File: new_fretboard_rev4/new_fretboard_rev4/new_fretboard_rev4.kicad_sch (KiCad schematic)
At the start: 48 parts, among them J1 Conn_01x06, J2 Conn_01x06, U1 LX3302AQPW_TSSOP-14, U2 LX3302AQPW_TSSOP-14

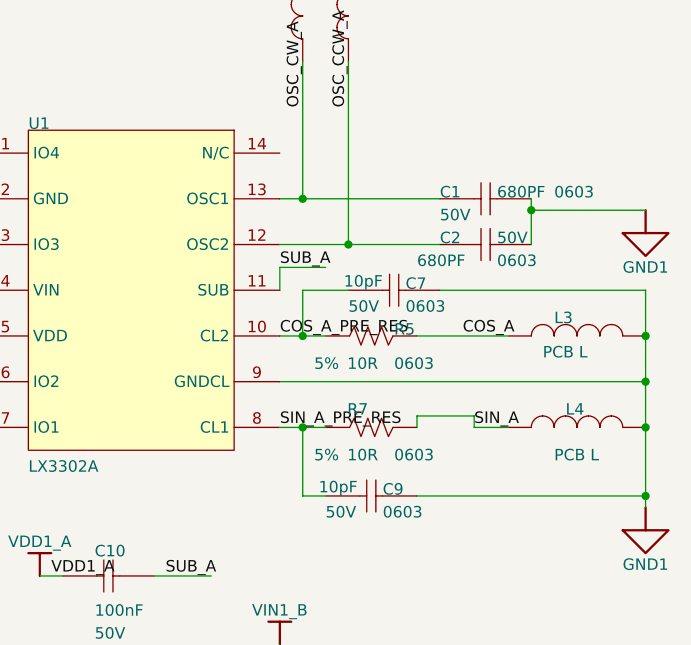
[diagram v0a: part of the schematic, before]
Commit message: partway through routing top
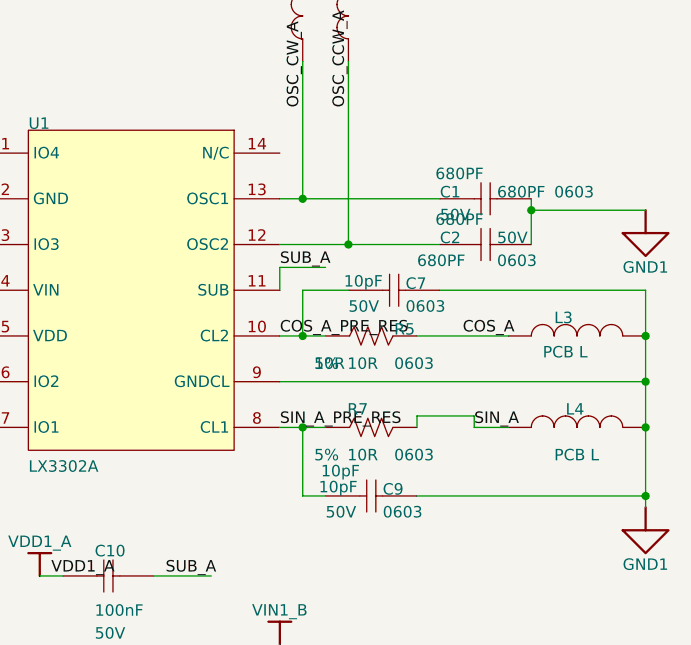
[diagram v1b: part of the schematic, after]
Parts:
- C1, C2, C21, C22: value Capacitor NP -> 680PF
- C10, C14, C18, C8: value Capacitor NP -> 100nF
- C11, C12, C13, C6: value Capacitor NP -> 6.8nF
- C15, C3: value Capacitor NP -> 1000pF
- C16, C4: value Capacitor NP -> 470nF
- C17, C5: value Capacitor NP -> 1uF
- C19, C20, C7, C9: value Capacitor NP -> 10pF
- R1, R8: value Resistor -> 221R
- R10, R2, R4, R9: value Resistor -> 10k
- R11, R6: value Resistor -> 4.7R
- R12, R13, R14, R3, R5, R7: value Resistor -> 10R
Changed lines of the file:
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@@
 			)
 		)
-		(property "Value" "Capacitor NP"
+		(property "Value" "680PF"
 			(at 200.152 76.708 0)
 			(effects
@@
 				)
 				(justify left bottom)
-				(hide yes)
 			)
 		)
@@
 			)
 		)
-		(property "Value" "Capacitor NP"
+		(property "Value" "6.8nF"
 			(at 53.848 184.912 0)
 			(effects
@@
 			)
 		)
-		(property "Value" "Capacitor NP"
+		(property "Value" "470nF"
 			(at 124.968 102.108 0)
 			(effects
@@
 			)
 		)
-		(property "Value" "Resistor"
+		(property "Value" "10R"
 			(at 184.15 203.2 0)
 			(effects
@@
 			)
 		)
-		(property "Value" "Capacitor NP"
+		(property "Value" "1uF"
 			(at 140.208 102.362 0)
 			(effects
@@
 			)
 		)
-		(property "Value" "Resistor"
+		(property "Value" "10k"
 			(at 96.52 75.692 0)
 			(effects
@@
 			)
 		)
-		(property "Value" "Capacitor NP"
+		(property "Value" "100nF"
 			(at 155.702 213.868 0)
 			(effects
@@
 			)
 		)
-		(property "Value" "Capacitor NP"
+		(property "Value" "6.8nF"
 			(at 76.708 184.912 0)
 			(effects
@@
 			)
 		)
-		(property "Value" "Capacitor NP"
+		(property "Value" "100nF"
 			(at 89.408 102.362 0)
 			(effects
@@
 			)
 		)
-		(property "Value" "Capacitor NP"
+		(property "Value" "6.8nF"
 			(at 56.388 89.662 0)
 			(effects
@@
 			)
 		)
-		(property "Value" "Capacitor NP"
+		(property "Value" "680PF"
 			(at 197.612 177.038 0)
 			(effects
@@
 			)
 		)
-		(property "Value" "Capacitor NP"
+		(property "Value" "6.8nF"
 			(at 79.248 89.662 0)
 			(effects
@@
 			)
 		)
-		(property "Value" "Resistor"
+		(property "Value" "4.7R"
 			(at 96.52 201.93 0)
 			(effects
@@
 			)
 		)
-		(property "Value" "Capacitor NP"
+		(property "Value" "10pF"
 			(at 189.992 86.868 0)
 			(effects
@@
 			)
 		)
-		(property "Value" "Resistor"
+		(property "Value" "10R"
 			(at 184.15 33.782 0)
 			(effects
@@
 			)
 		)
-		(property "Value" "Capacitor NP"
+		(property "Value" "100nF"
 			(at 158.242 118.618 0)
 			(effects
@@
 			)
 		)
-		(property "Value" "Resistor"
+		(property "Value" "10R"
 			(at 186.69 107.95 0)
 			(effects
@@
 			)
 		)
-		(property "Value" "Capacitor NP"
+		(property "Value" "1000pF"
 			(at 114.808 102.108 0)
 			(effects
@@
 			)
 		)
-		(property "Value" "Resistor"
+		(property "Value" "10R"
 			(at 181.61 129.032 0)
 			(effects
@@
 			)
 		)
-		(property "Value" "Capacitor NP"
+		(property "Value" "680PF"
 			(at 197.612 171.958 0)
 			(effects
@@
 			)
 		)
-		(property "Value" "Resistor"
+		(property "Value" "4.7R"
 			(at 99.06 106.68 0)
 			(effects
@@
 			)
 		)
-		(property "Value" "Resistor"
+		(property "Value" "221R"
 			(at 60.96 189.23 0)
 			(effects
@@
 			)
 		)
-		(property "Value" "Capacitor NP"
+		(property "Value" "10pF"
 			(at 187.452 109.728 0)
 			(effects
@@
 				)
 				(justify left bottom)
-				(hide yes)
 			)
 		)
@@
 			)
 		)
-		(property "Value" "Capacitor NP"
+		(property "Value" "1000pF"
 			(at 112.268 197.358 0)
 			(effects
@@
 			)
 		)
-		(property "Value" "Resistor"
+		(property "Value" "221R"
 			(at 63.5 93.98 0)
 			(effects
@@
 			)
 		)
-		(property "Value" "Resistor"
+		(property "Value" "10k"
 			(at 93.98 170.942 0)
 			(effects
@@
 			)
 		)
-		(property "Value" "Resistor"
+		(property "Value" "10R"
 			(at 184.15 193.04 0)
 			(effects
@@
 			)
 		)
-		(property "Value" "Capacitor NP"
+		(property "Value" "470nF"
 			(at 122.428 197.358 0)
 			(effects
@@
 			)
 		)
-		(property "Value" "Resistor"
+		(property "Value" "10R"
 			(at 186.69 97.79 0)
 			(effects
@@
 				)
 				(justify left bottom)
-				(hide yes)
 			)
 		)
@@
 			)
 		)
-		(property "Value" "Resistor"
+		(property "Value" "10k"
 			(at 86.36 75.692 0)
 			(effects
@@
 			)
 		)
-		(property "Value" "Capacitor NP"
+		(property "Value" "1uF"
 			(at 137.668 197.612 0)
 			(effects
@@
 			)
 		)
-		(property "Value" "Capacitor NP"
+		(property "Value" "100nF"
 			(at 86.868 197.612 0)
 			(effects
@@
 			)
 		)
-		(property "Value" "Capacitor NP"
+		(property "Value" "10pF"
 			(at 184.912 204.978 0)
 			(effects
@@
 			)
 		)
-		(property "Value" "Resistor"
+		(property "Value" "10k"
 			(at 83.82 170.942 0)
 			(effects
@@
 			)
 		)
-		(property "Value" "Capacitor NP"
+		(property "Value" "10pF"
 			(at 187.452 182.118 0)
 			(effects
@@
 			)
 		)
-		(property "Value" "Capacitor NP"
+		(property "Value" "680PF"
 			(at 200.152 81.788 0)
 			(effects
@@
 				)
 				(justify left bottom)
-				(hide yes)
 			)
 		)
